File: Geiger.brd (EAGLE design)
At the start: 137.1 x 47.9 mm, 41 parts, among them IC1 TINY15LS, IC3 TP4056, T1 BC807, T3 3904, T4 3904, T5 3904, U2 USB

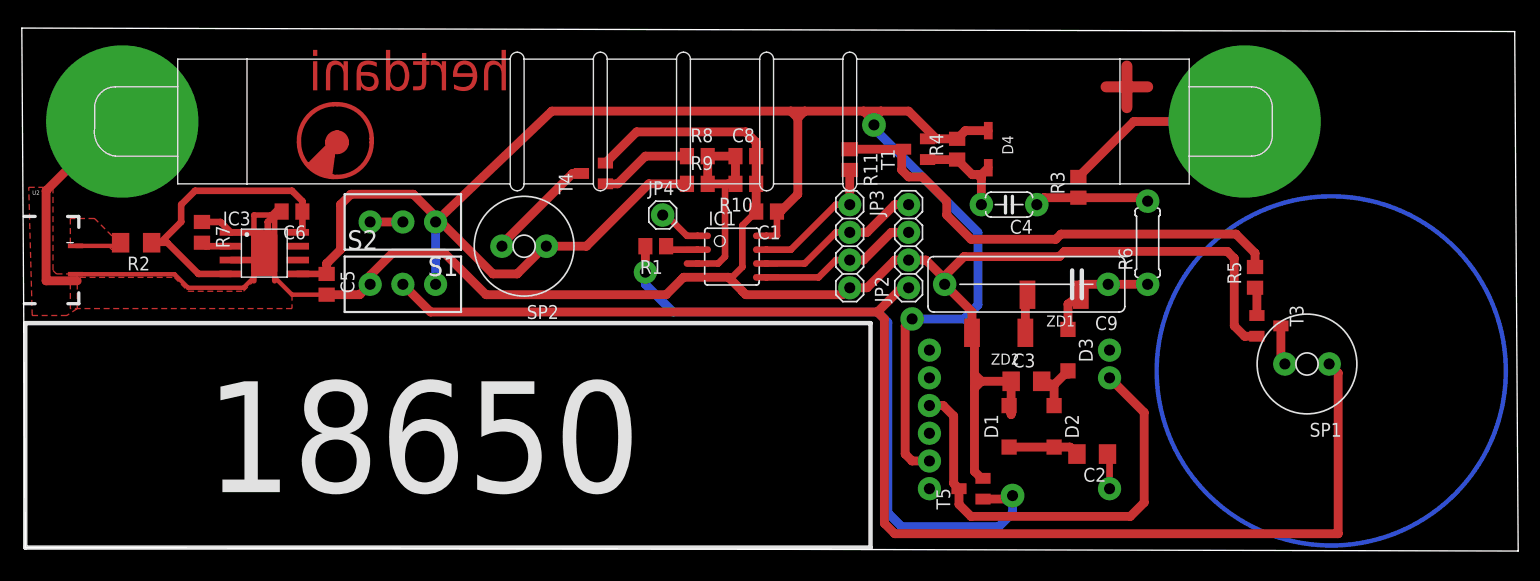
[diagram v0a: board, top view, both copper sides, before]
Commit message: dalsi
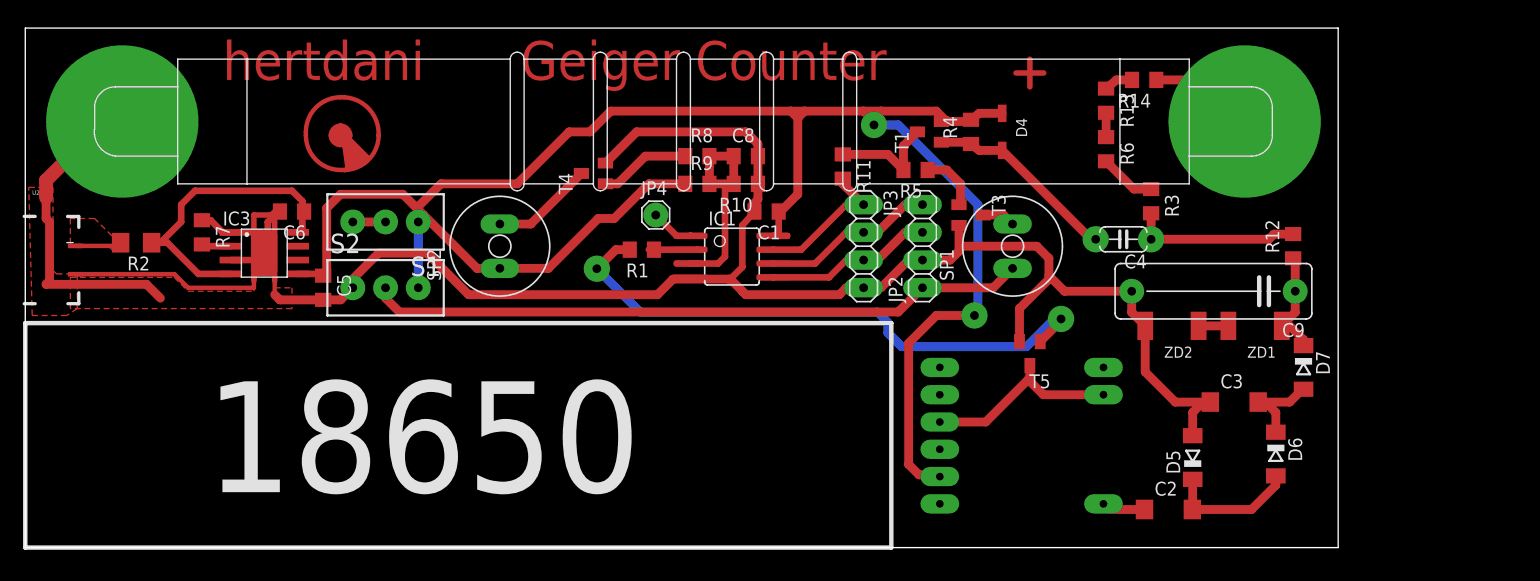
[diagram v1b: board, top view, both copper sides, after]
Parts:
- removed D1, D2, D3: BAV21W, diode:SOD123
- added D5, D6, D7: EGL1G, diode:SOD80C
- added R12, R13, R14: 1M, resistor:R0805
- R3: value 4M3 -> 1M
- R6: device resistor:0207/7 -> resistor:R0805
- moved R5 32.6 mm to (81.6, 34.6), turned to 180 degrees
- moved T3 29.1 mm to (86.7, 30.5)
- moved SP1 29.1 mm to (90.5, 27.6), turned to 90 degrees
- moved C3 19.1 mm to (110.8, 13.3)
- moved ZD1 18.6 mm to (112.7, 20.3)
- moved C9 17.2 mm to (108.9, 23.5)
- moved ZD2 15.9 mm to (105.1, 20.3)
- moved T5 13.5 mm to (92.1, 17.8), turned to 180 degrees
- moved C4 10.9 mm to (100.6, 28.3)
- moved R6 9.38 mm to (99.1, 36.5), turned to 270 degrees
- moved TRANSFORMER 9.26 mm to (83.8, 16.5)
- moved C2 8.64 mm to (104.8, 3.49), turned to 0 degrees
- moved R3 6.79 mm to (103.2, 31.8), turned to 270 degrees
- moved SP2 2.22 mm to (43.5, 27.6), turned to 90 degrees
- moved T1 2.03 mm to (82.9, 38.1)
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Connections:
- net VMEASURE renamed OSC
- removed net N$11: R3.2, U$1.P$1
- new net N$6: R3.1, R6.2
- new net N$7: R13.2, R6.1
- new net N$8: R14.1, U$1.P$1
- new net N$9: R13.1, R14.2
- net 200V2: now also D5.C, D6.A; no longer D1.C, D2.A
- net 400V: now also D7.C, R12.1; no longer D3.C, R6.1
- net 400V2: now also R12.2, R3.2; no longer R3.1, R6.2
- net 400V3: now also D6.C, D7.A; no longer D2.C, D3.A
- net GND: now also D5.A; no longer D1.A
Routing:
- net V+: track 125.8 -> 60.6 mm
- net N$10: track 44.9 -> 10.2 mm
- net N$18: track 41.6 -> 18.5 mm
- net N$11: track 17.3 -> 0.00 mm
- net N$8: track 0.00 -> 9.68 mm
- net N$12: track 9.28 -> 17.8 mm
- net N$4: track 62.0 -> 53.7 mm
- net VCC: track 171.5 -> 178.2 mm
- net 200V2: track 6.94 -> 12.4 mm
- net 400V2: track 10.6 -> 15.8 mm
- net N$6: track 0.00 -> 5.18 mm
- net GND: track 243.4 -> 238.6 mm
- net N$14: track 2.62 -> 5.51 mm
- net 400V3: track 5.22 -> 7.94 mm
- net N$9: track 0.00 -> 2.67 mm
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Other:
- board size 137.1 x 47.9 mm -> 120.3 x 47.6 mm
- board text added: "Geiger Counter"
